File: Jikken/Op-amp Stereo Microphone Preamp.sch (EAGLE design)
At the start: 29 parts, among them IC1 AD822N

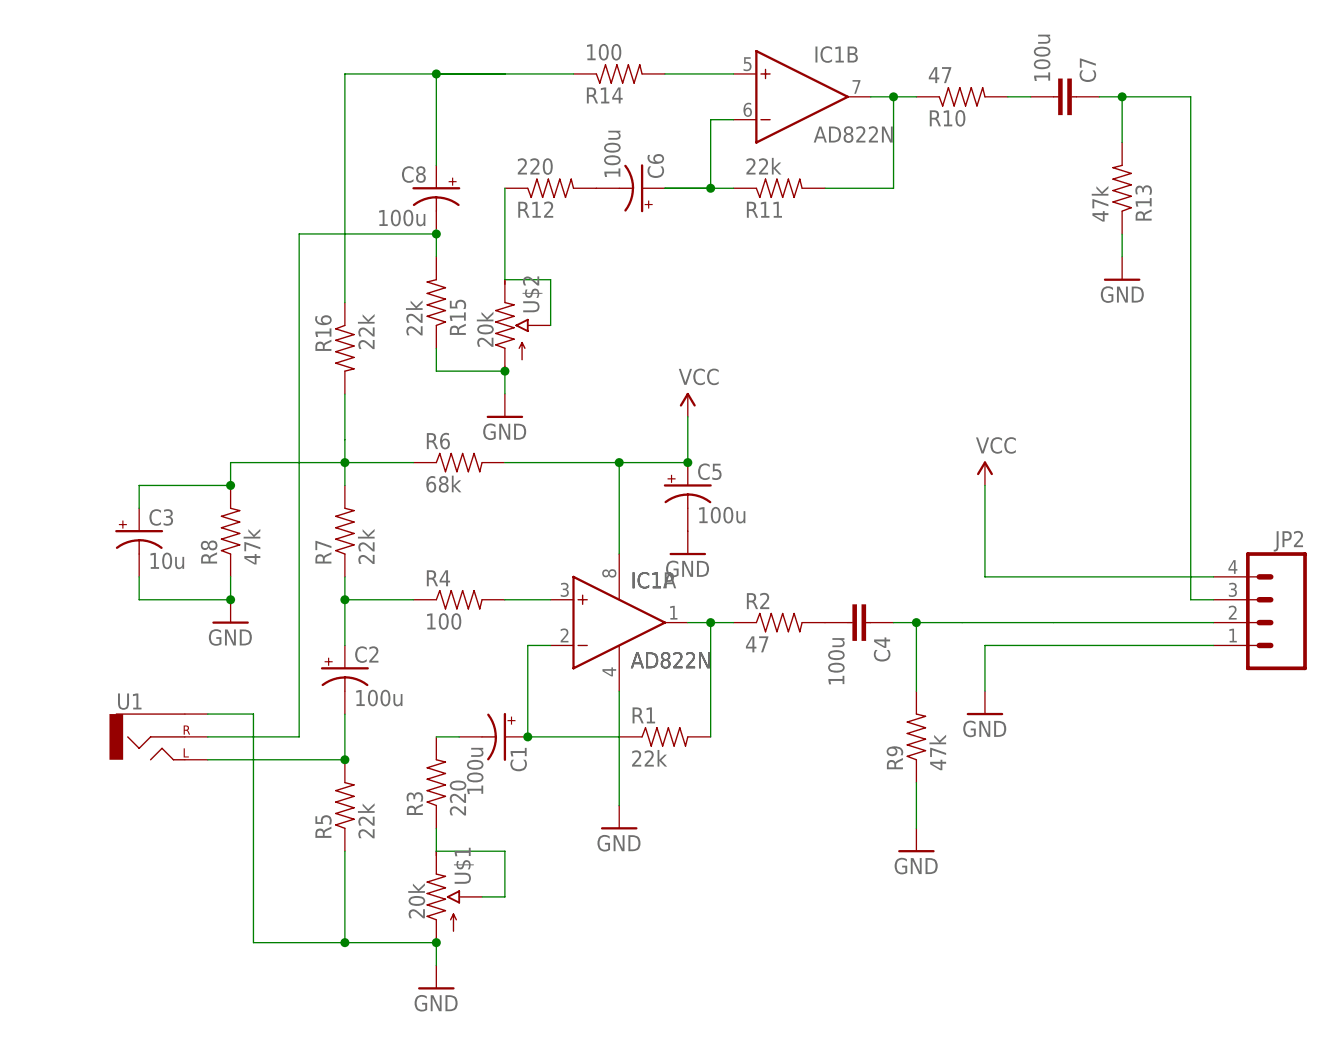
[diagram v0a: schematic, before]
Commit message: Amplifiers
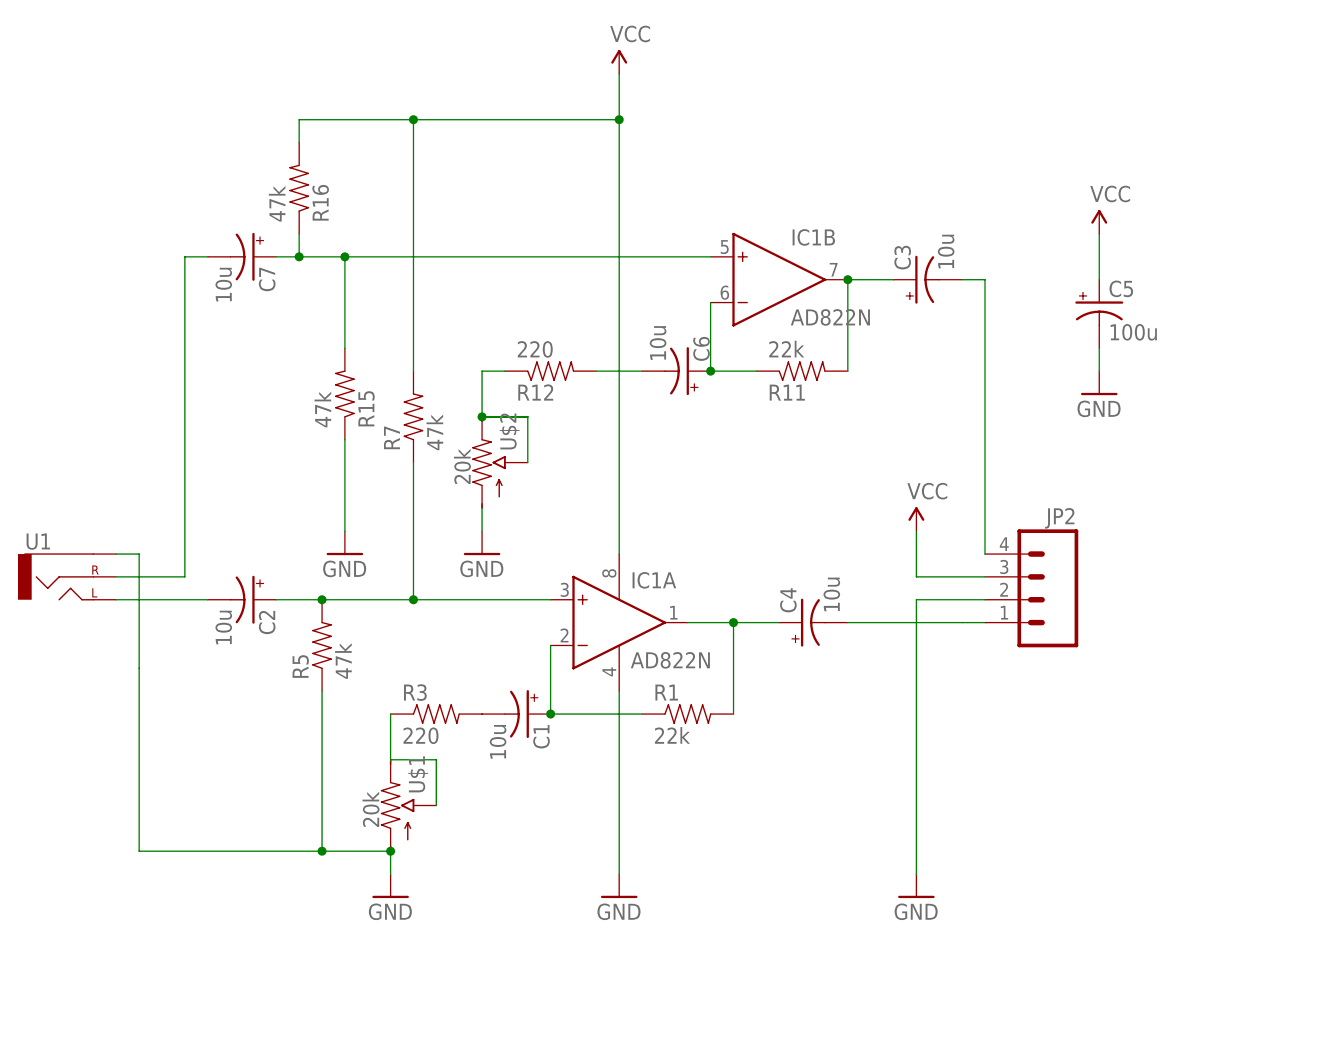
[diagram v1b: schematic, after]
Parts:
- removed C8: 100u, SparkFun:CAP_POLPTH1
- removed R10, R2: 47, My Library:RESISTORPTH-1/6W
- removed R13, R8, R9: 47k, My Library:RESISTORPTH-1/6W
- removed R14, R4: 100, My Library:RESISTORPTH-1/6W
- removed R6: 68k, My Library:RESISTORPTH-1/6W
- C1, C2, C6: value 100u -> 10u
- C4, C7: value 100u -> 10u; device capacitor-wima:C2.5/4 -> SparkFun:CAP_POLPTH1
- R11: device My Library:RESISTORPTH-1/6W -> SparkFun:RESISTORPTH-1/6W
- R12, R3: device My Library:RESISTORPTH-1/6W -> SparkFun:RESISTORPTH-1/4W
- R15, R5: value 22k -> 47k; device My Library:RESISTORPTH-1/6W -> SparkFun:RESISTORPTH-1/4W
- R16, R7: value 22k -> 47k; device My Library:RESISTORAXIAL-0.3 -> SparkFun:RESISTORPTH-1/4W
- U$1, U$2: device My Library:POT-RV16AF-20 -> My Library:POT100K_3362U
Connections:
- removed net N$15: C8.-, R15.2, U1.RIGHT
- removed net N$16: C7.2, R10.2
- removed net N$17: C7.1, JP2.3, R13.2
- removed net N$18: C8.+, R14.1, R16.1
- removed net N$19: IC1B.IN+, R14.2
- net GND: now also JP2.2; no longer C3.-, JP2.1, R13.1, R8.1, R9.1
- net N$13: now also C4.-, JP2.1; no longer C4.1, JP2.2, R9.2
- net N$14: now also C3.+; no longer R10.1
- net N$3: now also C4.+; no longer R2.1
- net N$4: now also C3.-, JP2.4; no longer C4.2, R2.2
- net N$6: now also C2.+, IC1A.IN+, R7.1; no longer C2.-, U1.LEFT
- net N$7: now also C7.+, IC1B.IN+, R15.2, R16.1; no longer C2.+, R4.1, R7.1
- net N$8: now also C2.-, U1.LEFT; no longer IC1A.IN+, R4.2
- net N$9: now also C7.-, U1.RIGHT; no longer C3.+, R16.2, R6.1, R7.2, R8.2
- net VCC: now also JP2.3, R16.2, R7.2; no longer JP2.4, R6.2
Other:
- moved on the sheet: C1, C2, C3, C5, C6, IC1B, JP2, R1, R11, R12, R15, R16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
